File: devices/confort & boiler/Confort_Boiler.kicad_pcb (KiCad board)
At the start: 2 copper layers, 25 parts, among them K1 DHT1, K2 DHT2, K3 DS18B20, P1 TOBOILER, Q1 BC558, U1 OPTO-TRANSISTOR4, U2 ARDUINO_MINI, U3 ENC28J60, U4 OPTO-TRANSISTOR4

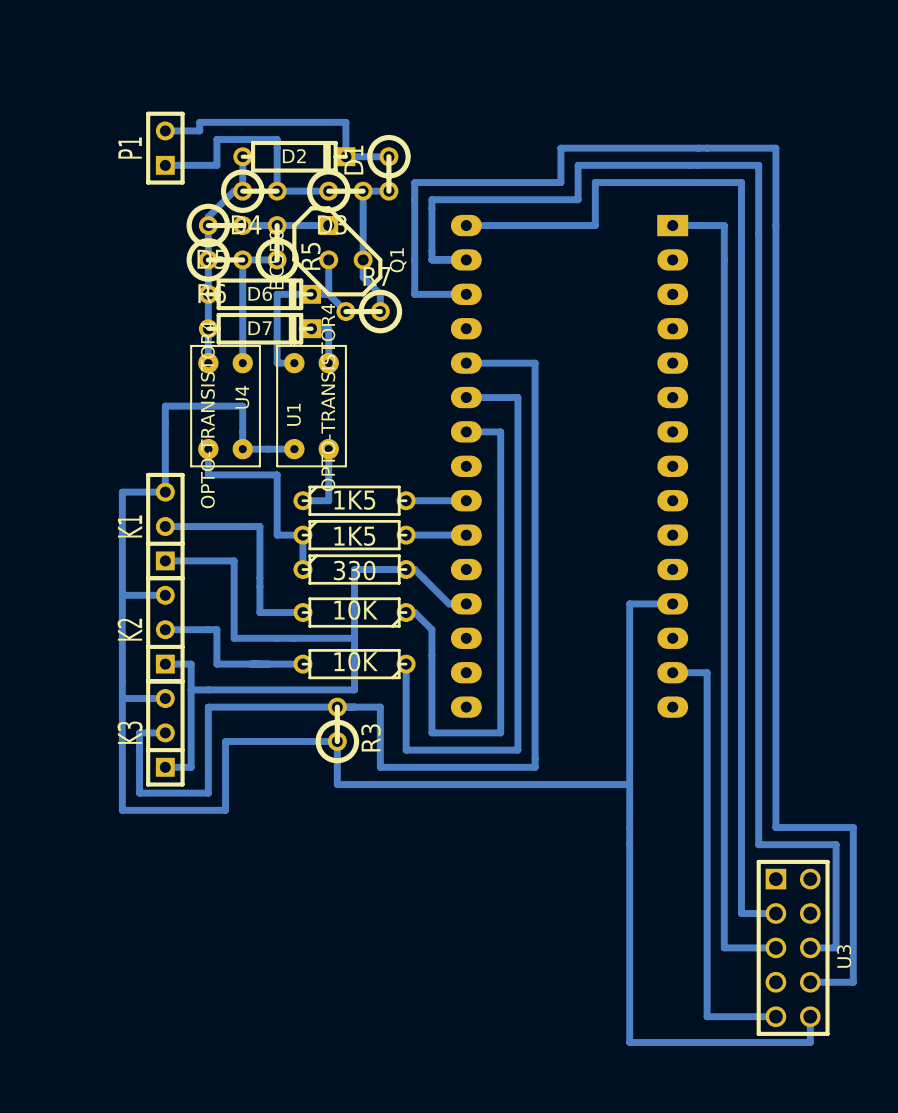
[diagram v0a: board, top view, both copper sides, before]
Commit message: finished with pcb
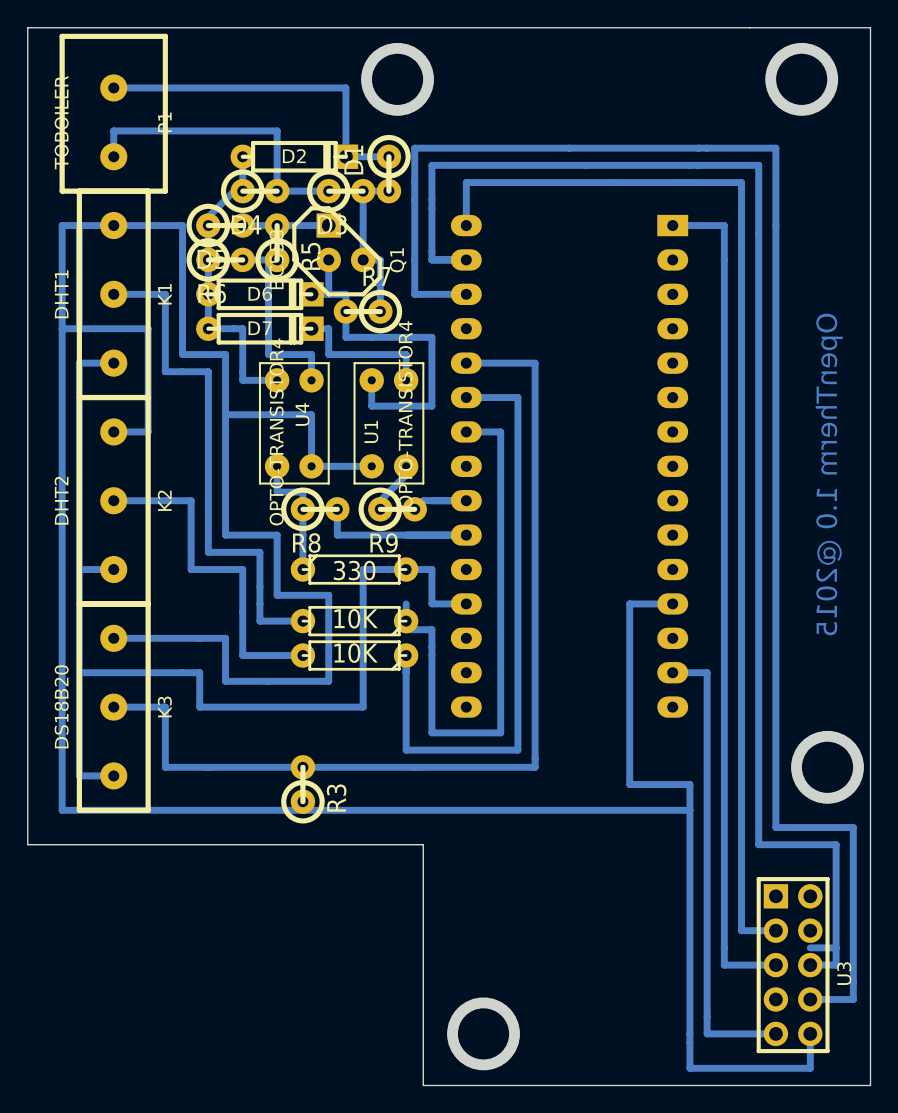
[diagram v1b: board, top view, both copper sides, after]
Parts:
- K1, K2, K3: footprint SIL-3 -> DG306-5.08-03
- P1: footprint SIL-2 -> DG306-5.08-02
- R8, R9: footprint R3 -> R1
- moved K1 17.6 mm to (99.7, 35.6)
- moved K2 10.3 mm to (99.7, 50.8)
- moved U1 5.85 mm to (120.0, 44.5)
- moved U4 5.24 mm to (113.0, 45.7)
- moved R3 5.12 mm to (113.7, 71.8)
- moved P1 4.26 mm to (99.7, 22.9)
- moved K3 4.26 mm to (99.7, 66.0)
- moved R9 3.24 mm to (120.7, 51.4)
- moved R8 3.17 mm to (114.9, 51.4)
- moved U3 1.27 mm to (149.9, 85.1)
- moved R2 0.64 mm to (117.5, 62.2)
- moved R1 0.63 mm to (117.5, 59.7)
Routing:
- net VCC: track 148.6 -> 254.0 mm
- net GND: track 94.4 -> 116.2 mm
- net N-0000010: track 16.5 -> 38.1 mm
- net LDS18B20: track 83.2 -> 70.5 mm
- net N-0000023: track 14.5 -> 26.0 mm
- net LRX: track 4.45 -> 15.9 mm
- net N-0000013: track 14.6 -> 25.4 mm
- net N-0000018: track 3.81 -> 10.8 mm
- net N-0000022: track 16.7 -> 23.0 mm
- net N-0000016: track 15.9 -> 9.53 mm
- net N-000009: track 19.7 -> 25.4 mm
- net N-0000017: track 10.2 -> 15.2 mm
- net N-0000019: track 17.8 -> 22.2 mm
- net N-000003: track 101.6 -> 104.8 mm
- net LTX: track 4.45 -> 6.61 mm
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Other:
- board outline added: 62.2 x 78.1 mm
- board text added: "OpenTherm 1.0 @2015"
